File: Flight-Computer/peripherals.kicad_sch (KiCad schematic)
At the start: 36 parts, among them P10 Micro_SD_Card, P8 USB, P9 1984659, Q5 QS5U17TR, Q6 QS5U17TR, U10 TS391IYLT, U11 TS391IYLT, U6 SST25VF040B-50-4I-S2AE-T, U7 RFM95W-868S2, U8 CP2102-GMR(QFN28), U9 TS391IYLT

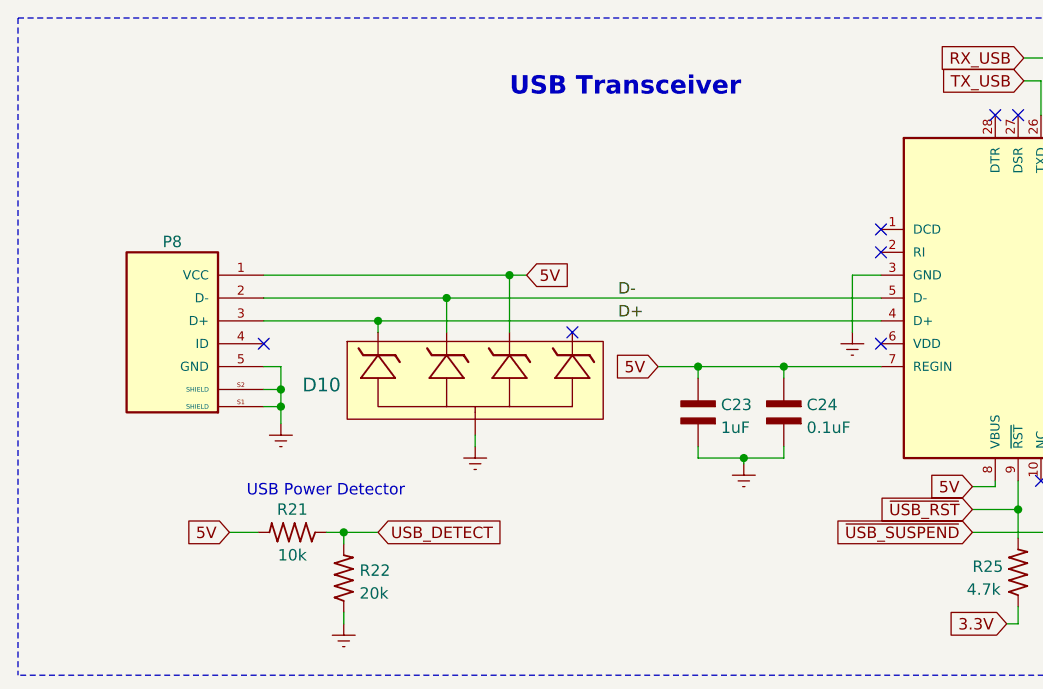
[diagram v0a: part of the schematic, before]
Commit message: Add files via upload
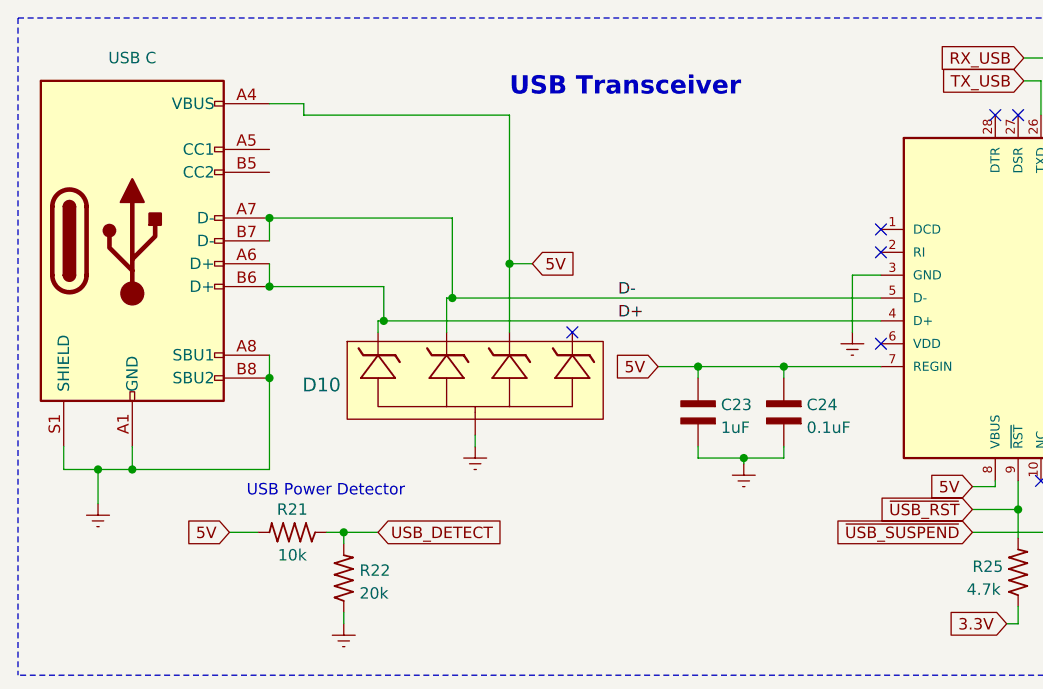
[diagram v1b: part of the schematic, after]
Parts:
- removed P8: USB, Flight-Computer:10118194-0001LF, symbol Flight-Computer:USB
- added J: USB C, symbol Connector:USB_C_Receptacle_USB2.0_16P
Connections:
- net 5V: now also J.A4 (VBUS), J.A9 (VBUS), J.B4 (VBUS), J.B9 (VBUS)
- net D+: now also J.A6 (D+), J.B6 (D+)
- net D-: now also J.A7 (D-), J.B7 (D-)
- net Earth: now also J.A1 (GND), J.A12 (GND), J.A8 (SBU1), J.B1 (GND), J.B12 (GND), J.B8 (SBU2), J.S1 (SHIELD)
- no-connect marks 21 -> 20
